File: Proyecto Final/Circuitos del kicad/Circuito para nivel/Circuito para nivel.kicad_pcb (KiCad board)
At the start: 2 copper layers, 50.1 x 30 mm, 10 parts, among them J1 Conn_01x05, J2 Conn_01x03, Q1 2N3904, Q2 2N3904, Q3 2N3904, Q4 2N3904

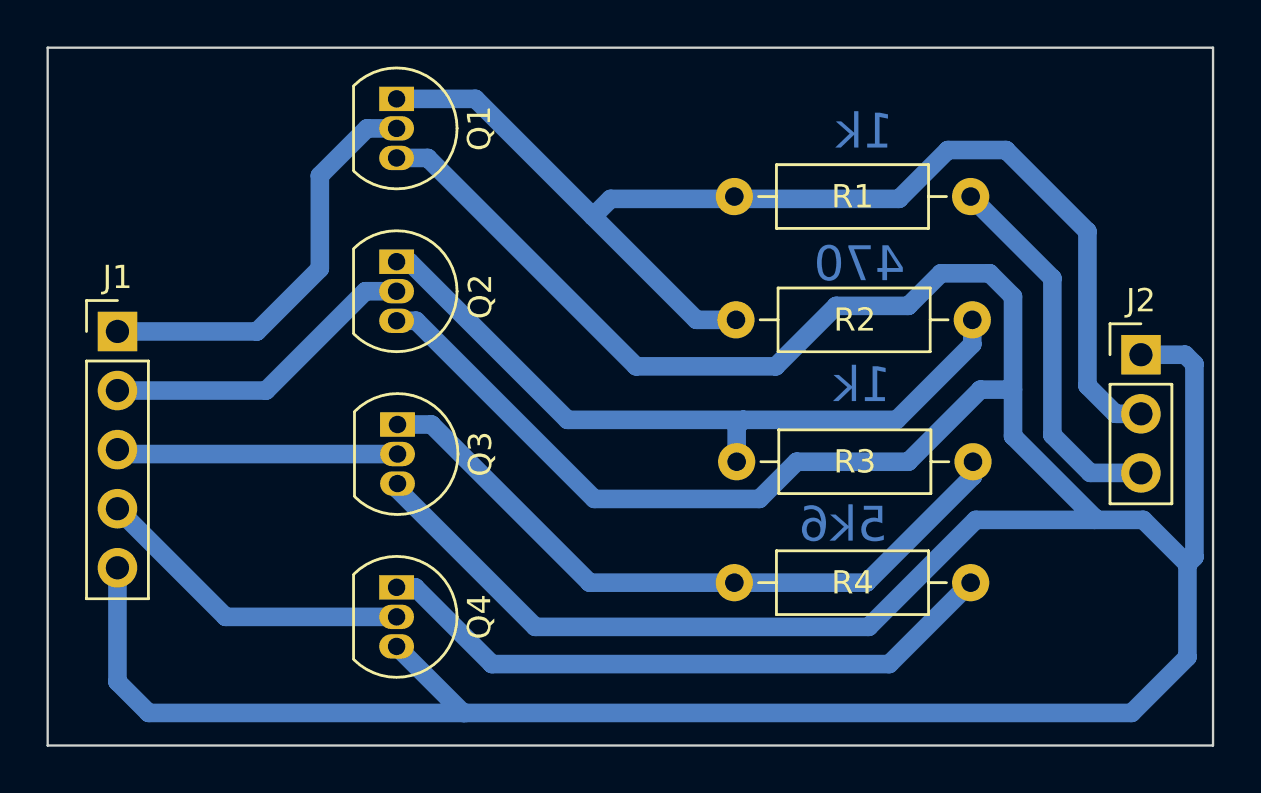
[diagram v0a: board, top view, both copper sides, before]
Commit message: cum
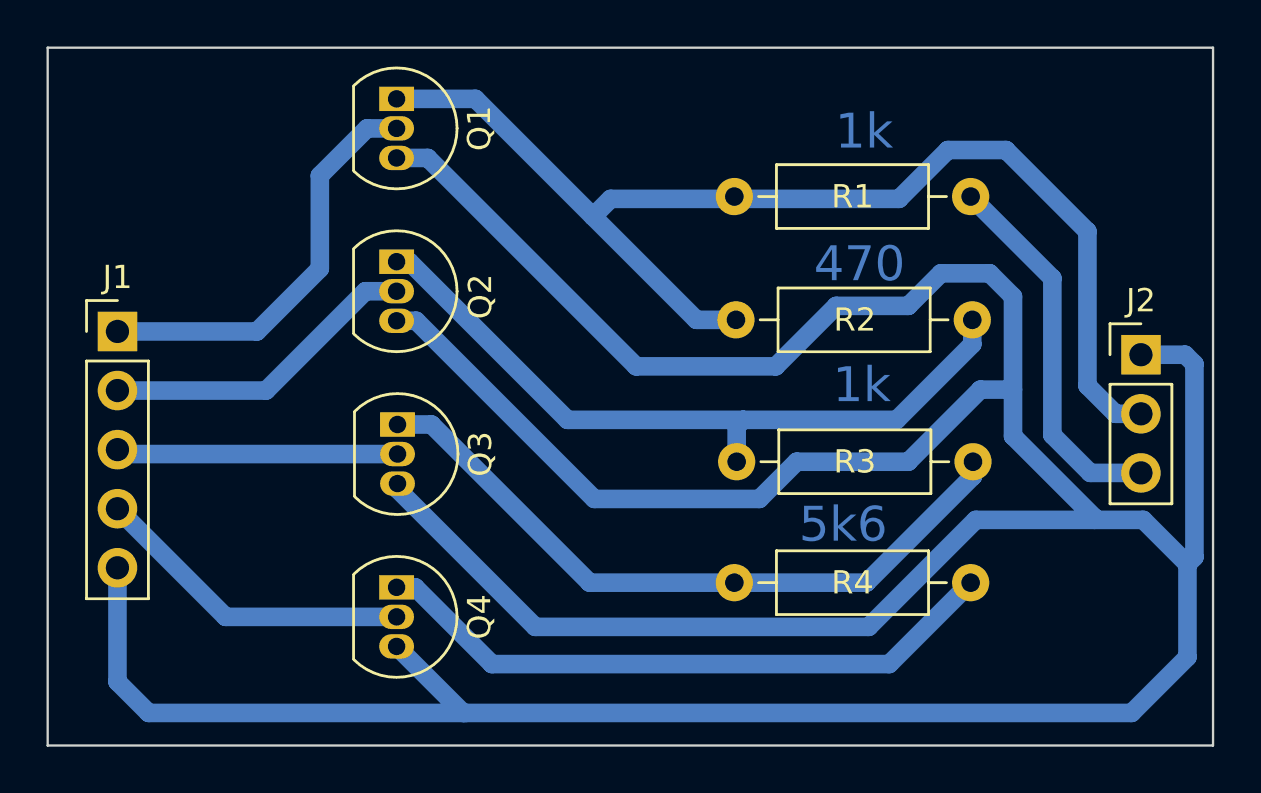
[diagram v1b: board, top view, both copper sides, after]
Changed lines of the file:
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@@
     ) (layer "Edge.Cuts") (width 0.1) (fill none))
   (gr_text "470" (at 149.9 71.1) (layer "B.Cu")
-    (effects (font (size 1.5 1.5) (thickness 0.3)) (justify mirror))
+    (effects (font (size 1.5 1.5) (thickness 0.3)))
   )
   (gr_text "1k\n" (at 150 76.3) (layer "B.Cu")
-    (effects (font (size 1.5 1.5) (thickness 0.3)) (justify mirror))
+    (effects (font (size 1.5 1.5) (thickness 0.3)))
   )
   (gr_text "1k\n" (at 150.1 65.4) (layer "B.Cu")
-    (effects (font (size 1.5 1.5) (thickness 0.3)) (justify mirror))
+    (effects (font (size 1.5 1.5) (thickness 0.3)))
   )
   (gr_text "5k6\n" (at 149.2 82.3) (layer "B.Cu")
-    (effects (font (size 1.5 1.5) (thickness 0.3)) (justify mirror))
+    (effects (font (size 1.5 1.5) (thickness 0.3)))
   )
   (segment (start 130 66.54) (end 131.34 66.54) (width 0.8) (layer "B.Cu") (net 1))
